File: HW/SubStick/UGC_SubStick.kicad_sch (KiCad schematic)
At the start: 1 part, among them SW1 GL18_SW

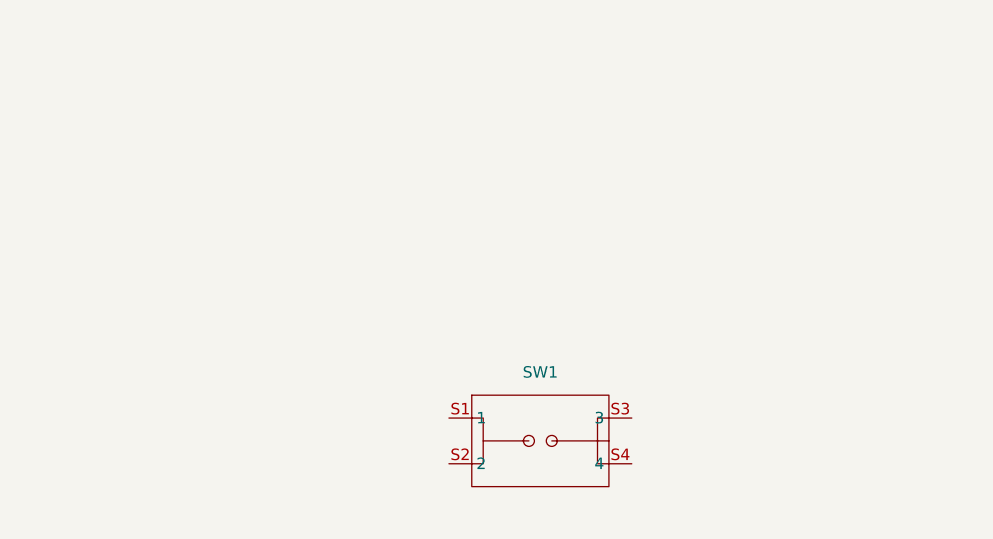
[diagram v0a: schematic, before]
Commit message: Updates
- Stick PCB
- USB C pcb
- trigger PCB
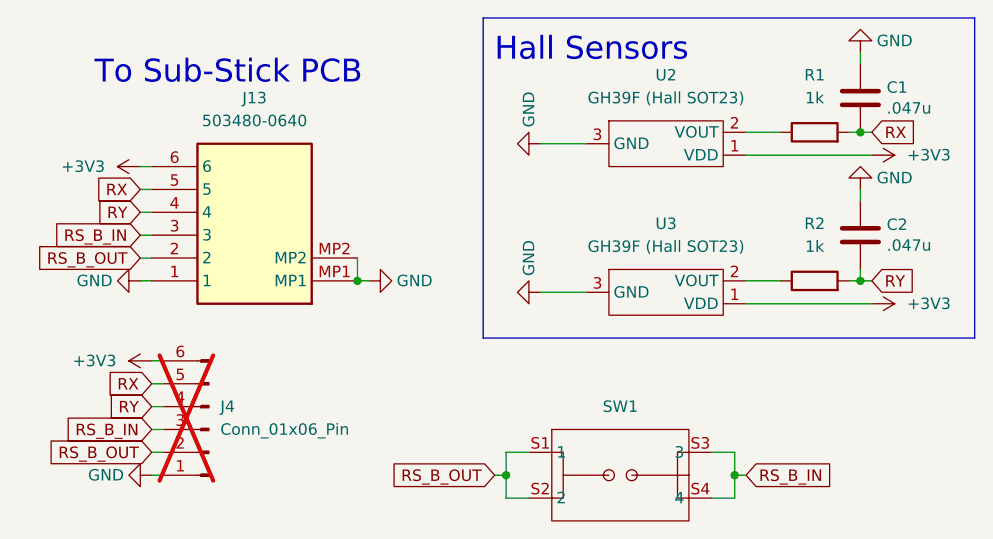
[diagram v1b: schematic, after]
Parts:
- added C1, C2: .047u, Capacitor_SMD:C_0603_1608Metric_Pad1.08x0.95mm_HandSolder, symbol Device:C
- added J13: 503480-0640, hhl:5034800640, symbol hhl:503480-0640
- added J4: Conn_01x06_Pin, Connector_PinHeader_2.00mm:PinHeader_1x06_P2.00mm_Vertical, symbol Connector:Conn_01x06_Pin
- added R1, R2: 1k, Resistor_SMD:R_0201_0603Metric, symbol Device:R
- added U2, U3: GH39F (Hall SOT23), hhl:GH39F, symbol progcc_v3:GH39F (Hall SOT23)
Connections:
- net RS_B_OUT: now reaches SW1.S1 (1)
- net RS_B_OUT: now also SW1.S2 (2), J13.2, J4.2 (Pin_2)
- net RS_B_IN: now reaches SW1.S3 (3)
- net RS_B_IN: now also SW1.S4 (4), J13.3, J4.3 (Pin_3)
- new net: R1.1, U2.2 (VOUT)
- new net: R2.1, U3.2 (VOUT)
- new net +3V3: J13.6, J4.6 (Pin_6), U2.1 (VDD), U3.1 (VDD)
- new net GND: C1.1, C2.1, J13.1, J13.MP1, J13.MP2, J4.1 (Pin_1), U2.3 (GND), U3.3 (GND)
- new net RX: C1.2, J13.5, J4.5 (Pin_5), R1.2
- new net RY: C2.2, J13.4, J4.4 (Pin_4), R2.2
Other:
- note added: "Hall Sensors"
- note added: "To Sub-Stick PCB"
- moved on the sheet: SW1

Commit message: Production files
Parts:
- J13: MPN (none) -> 503480-0640; Manufacturer_Part_Number 503480-0640 -> (none)
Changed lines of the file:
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@@
       (effects (font (size 1.27 1.27)) (justify left top) hide)
     )
-    (property "Manufacturer_Part_Number" "503480-0640" (at 195.58 -660.3 0)
+    (property "MPN" "503480-0640" (at 195.58 -660.3 0)
       (effects (font (size 1.27 1.27)) (justify left top) hide)
     )

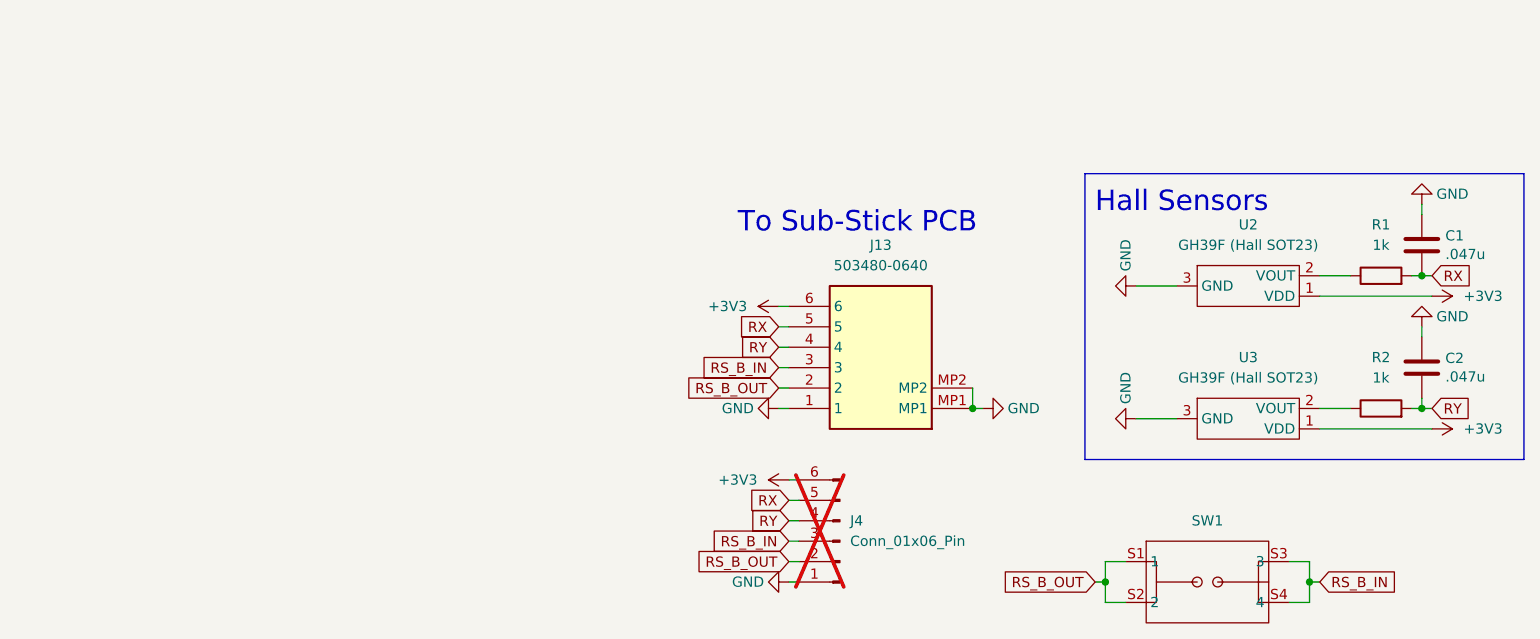
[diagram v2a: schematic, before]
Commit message: R4 updates to hardware
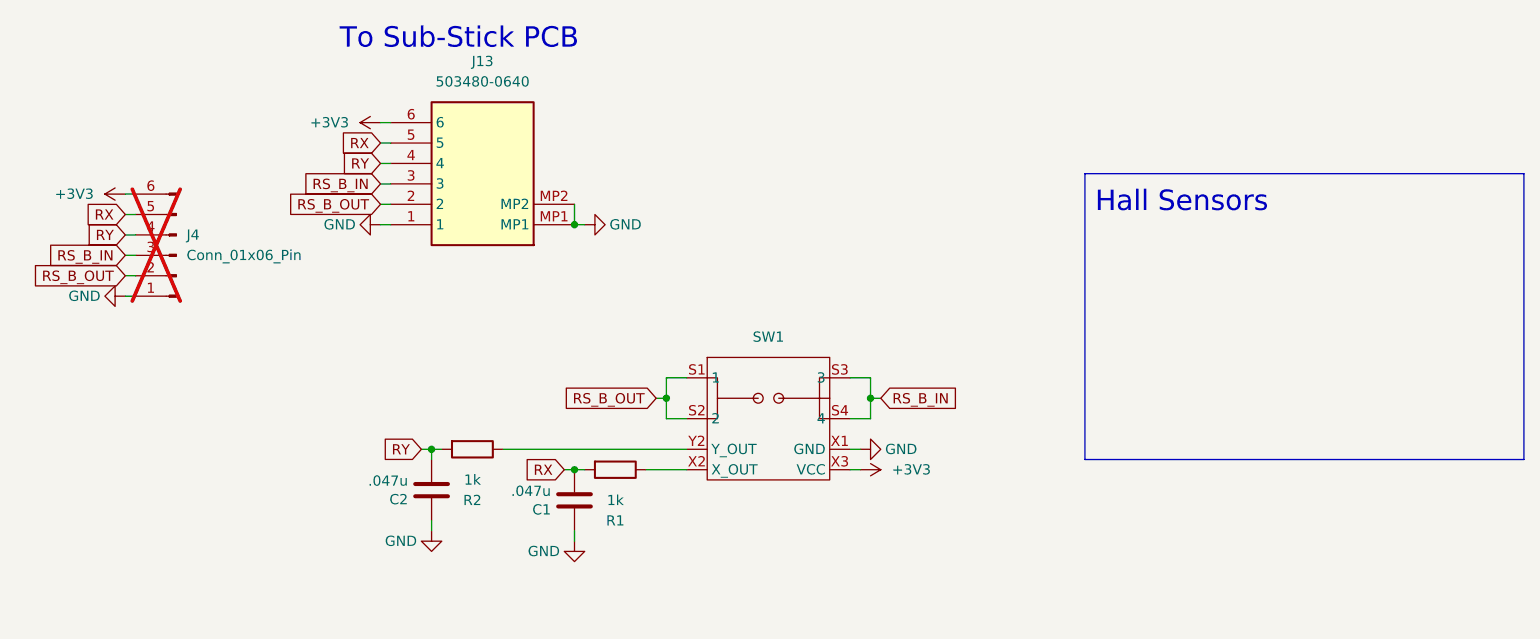
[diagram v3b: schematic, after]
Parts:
- removed U2, U3: GH39F (Hall SOT23), hhl:GH39F, symbol progcc_v3:GH39F (Hall SOT23)
- SW1: footprint hhl:GL18 -> hhl:GL1807SYAE; symbol hhl:GL18_SW -> hhl:GL1807SYAE-002; MPN GL18 -> GL1807SYAE-002
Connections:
- net +3V3: now also SW1.X3 (VCC), SW1.Y3 (VCC)
- net GND: now also SW1.X1 (GND), SW1.Y1 (GND)
- net at R1.1: now also SW1.X2 (X_OUT)
- net at R2.1: now also SW1.Y2 (Y_OUT)
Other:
- moved on the sheet: C1, C2, J13, J4, R1, R2
